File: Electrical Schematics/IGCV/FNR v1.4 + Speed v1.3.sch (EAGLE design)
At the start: 40 parts, among them IC3 DPOT, K1 DF2-L-DC24V, K2 35701331, K3 35701331, K4 G6C-2117P, K5 35701331, Q1 BUZ11, Q2 BUZ11, Q3 BUZ11, SW2 Pedal MS, SW3 Pedal MS, SW4 E-STOP, SW5 TVS, SW6 KEY

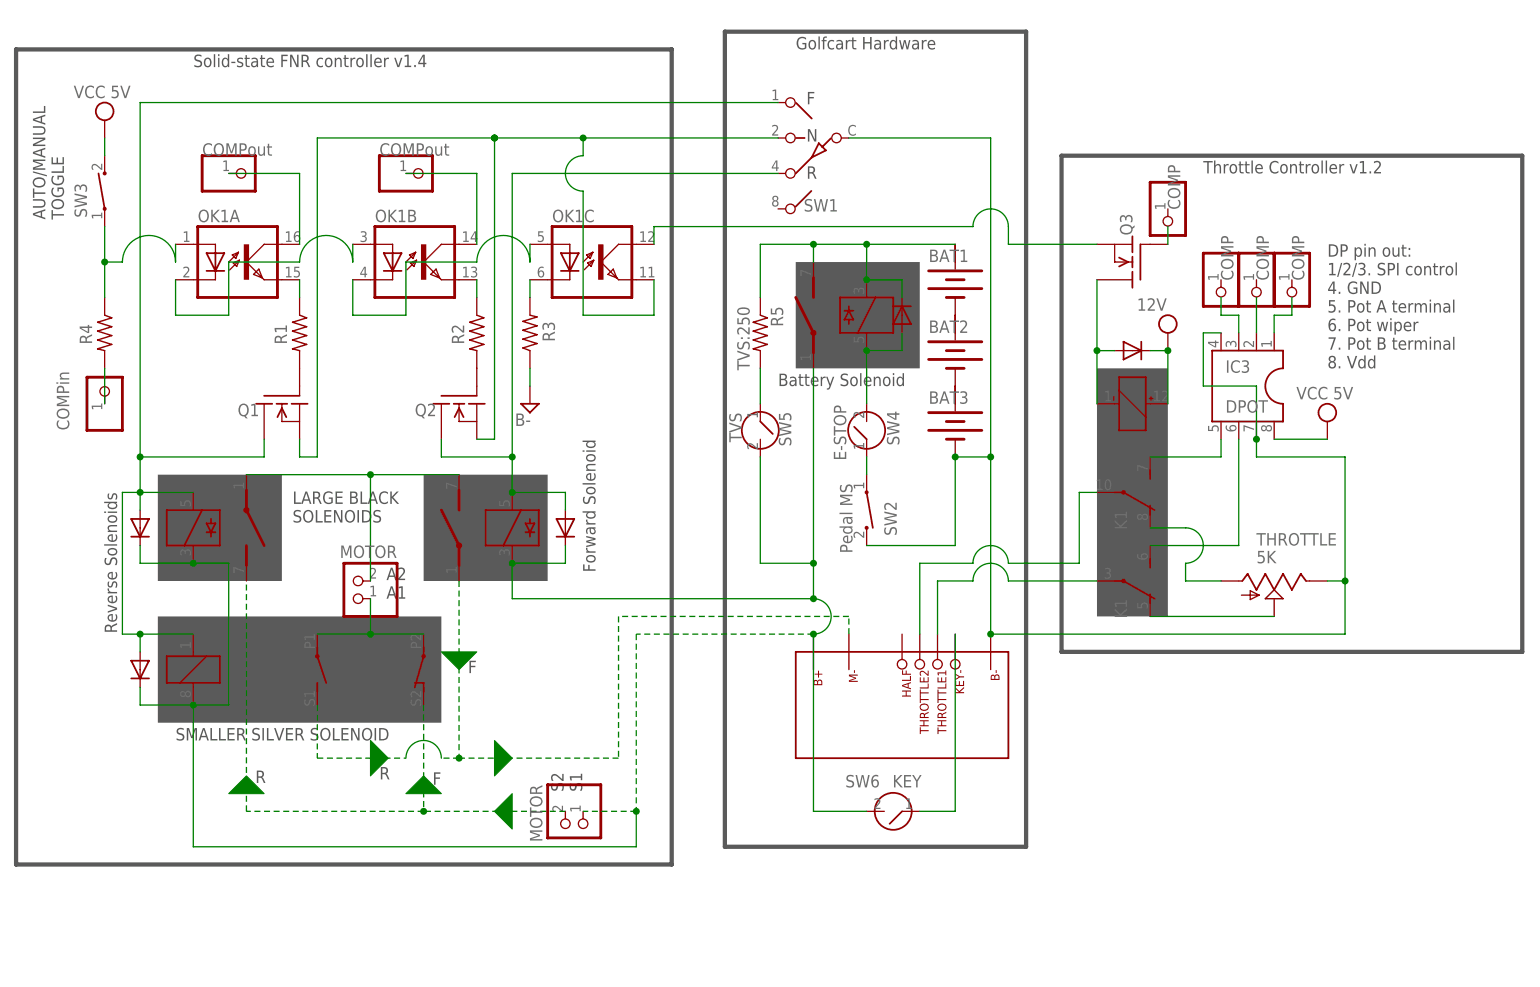
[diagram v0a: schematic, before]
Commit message: updated schematic
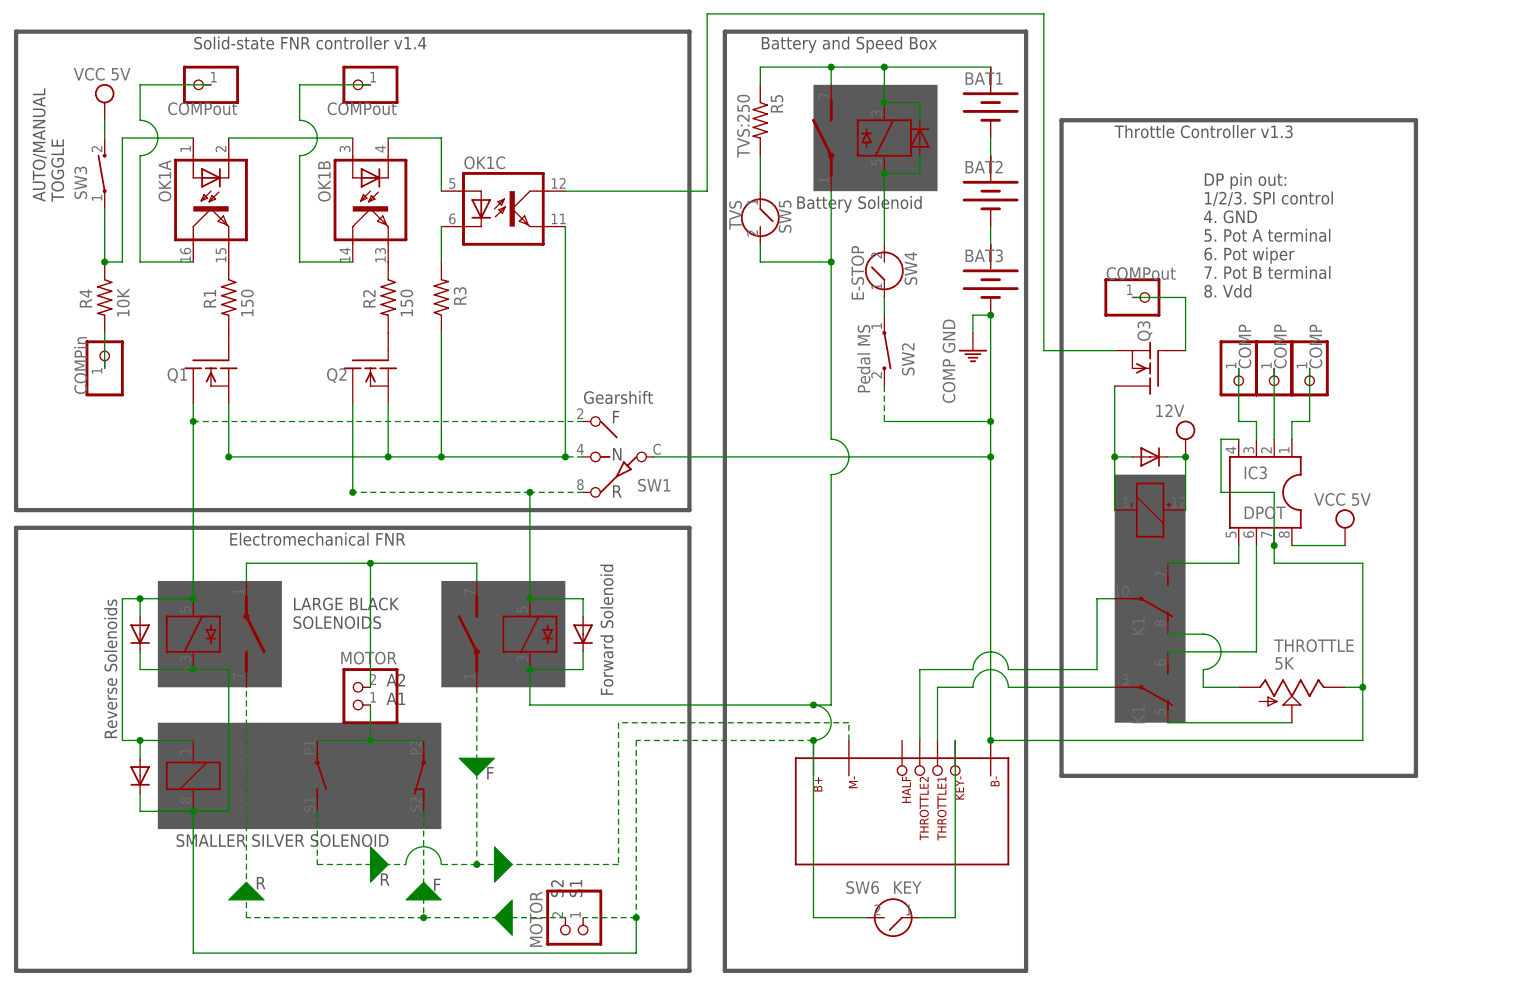
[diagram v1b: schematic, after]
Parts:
- JP37: value COMP -> COMPout
- R1, R2: value (none) -> 150
- R4: value (none) -> 10K
- SW1: device special:SW-C10 -> custom:SW-1P3T
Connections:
- removed net GND1: R3.1
- new net PE: BAT3.-, IC3.4, IC3.7, SW1.C, SW2.2, THROTTLE.E, U$5.B-
- net B-: now also R3.1; no longer BAT3.-, IC3.4, IC3.7, SW1.C, SW2.2, THROTTLE.E, U$5.B-
- net N$117: now also JP35.1
- net N$118: now also JP36.1
- net N$119: now also JP34.1
- net N$121: now also JP37.1
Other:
- note added: "Battery and Speed Box"
- note added: "Electromechanical FNR"
- note added: "Gearshift"
- note added: "Throttle Controller v1.3"
- note removed: "Golfcart Hardware"
- note removed: "Throttle Controller v1.2"
- moved on the sheet: BAT1, BAT2, BAT3, IC3, K1, OK1A, OK1B, OK1C, Q1, Q2, Q3, R1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
